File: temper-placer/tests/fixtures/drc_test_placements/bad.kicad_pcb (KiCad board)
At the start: 2 copper layers, 50 x 30 mm, 4 parts, among them U1 LM358

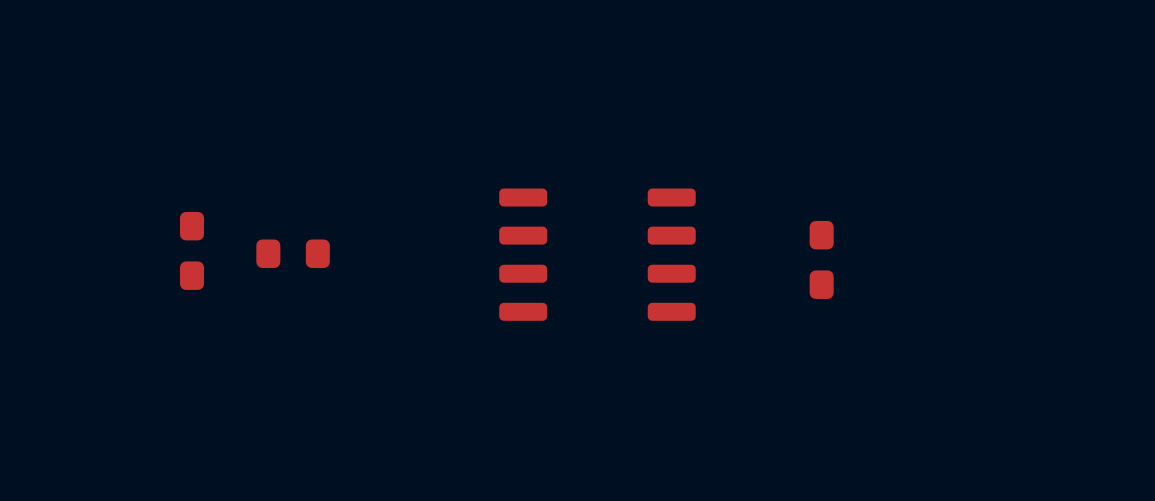
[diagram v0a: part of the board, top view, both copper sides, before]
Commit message: merge for sharing
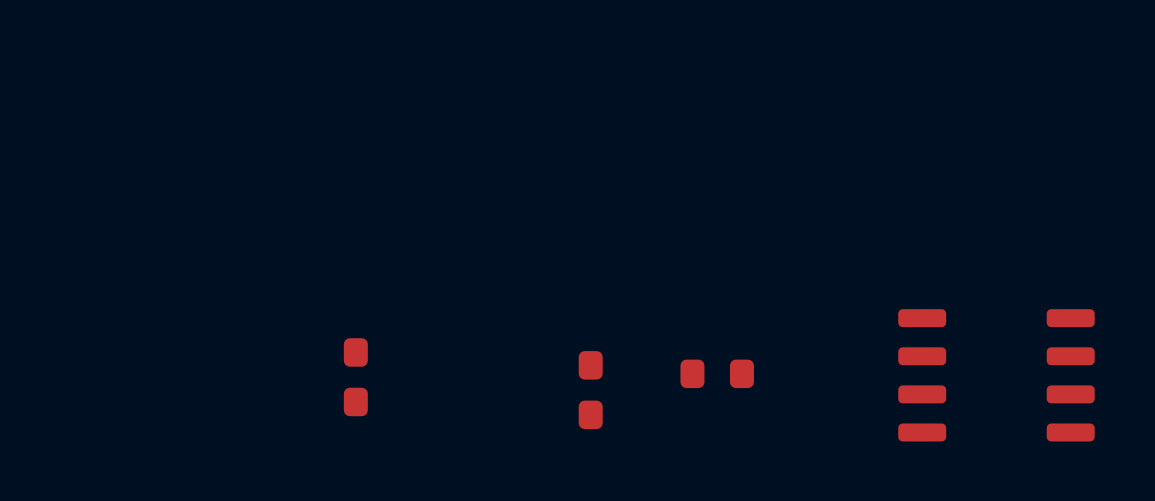
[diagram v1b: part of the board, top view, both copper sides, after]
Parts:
- moved R1 18.0 mm to (207.7, 158.0), turned to 0 degrees
- moved C1 16.0 mm to (195.6, 158.1)
- moved U1 13.9 mm to (217.0, 158.0)
- moved R2 10.9 mm to (203.5, 158.5), turned to 90 degrees
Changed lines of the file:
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@@
   (net 4 "SIG2")
   (footprint "Resistor_SMD:R_0603_1608Metric" (layer "F.Cu")
-    (at 190.17899923476529 153.88604800885992 90.0)
+    (at 207.68600773709272 157.98380544119928 0.0)
     (property "Reference" "R1")
     (property "Value" "10k")
@@
   )
   (footprint "Resistor_SMD:R_0603_1608Metric" (layer "F.Cu")
-    (at 193.54858199234525 153.97999831282684 0.0)
+    (at 203.4687740581351 158.525071262886 90.0)
     (property "Reference" "R2")
     (property "Value" "4.7k")
@@
   )
   (footprint "Capacitor_SMD:C_0603_1608Metric" (layer "F.Cu")
-    (at 211.16778503982619 154.18675466308457 270.0)
+    (at 195.64002169838204 158.0957986818985 270.0)
     (property "Reference" "C1")
     (property "Value" "100nF")
@@
   )
   (footprint "Package_SO:SOIC-8_3.9x4.9mm_P1.27mm" (layer "F.Cu")
-    (at 203.69531233817753 154.01117744176125 0.0)
+    (at 216.9941903301225 158.03294687515967 0.0)
     (property "Reference" "U1")
     (property "Value" "LM358")
